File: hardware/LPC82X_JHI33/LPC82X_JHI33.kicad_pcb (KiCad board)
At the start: 2 copper layers, 23.6 x 23.5 mm, 24 parts, among them J1 LPC82XJHI33_LEFT, J2 LPC82XJHI33_RIGHT, J3 JTAG_2X05, U1 LPC824M201JHI33, Y1 12MHz

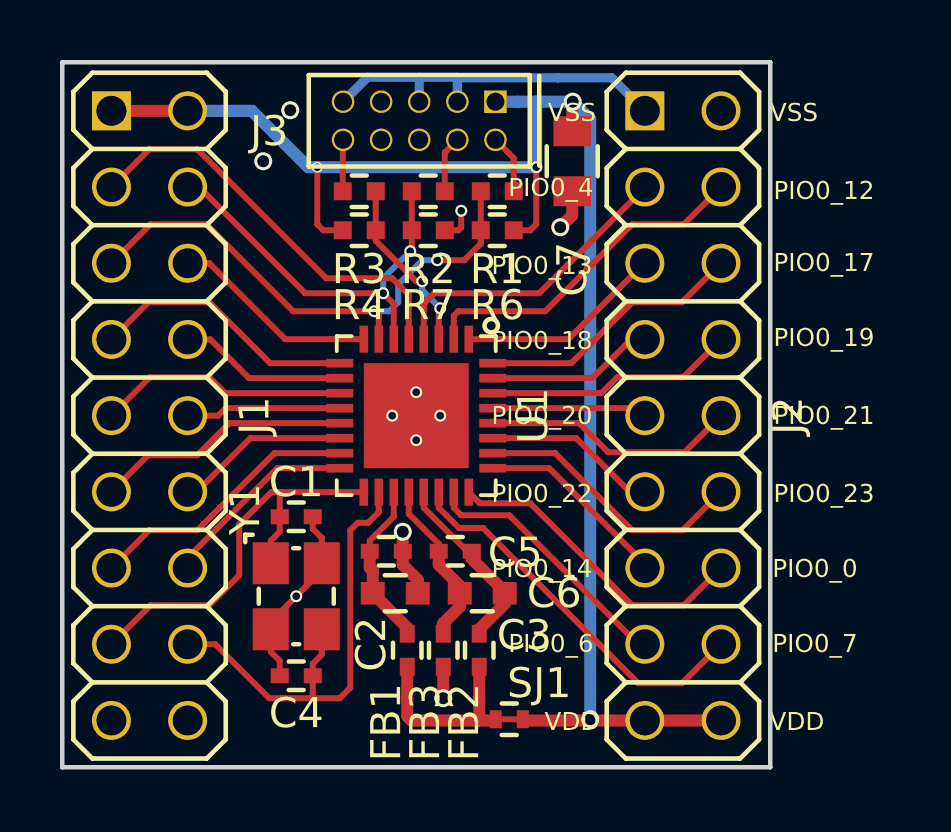
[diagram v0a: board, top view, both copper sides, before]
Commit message: silk placement completed
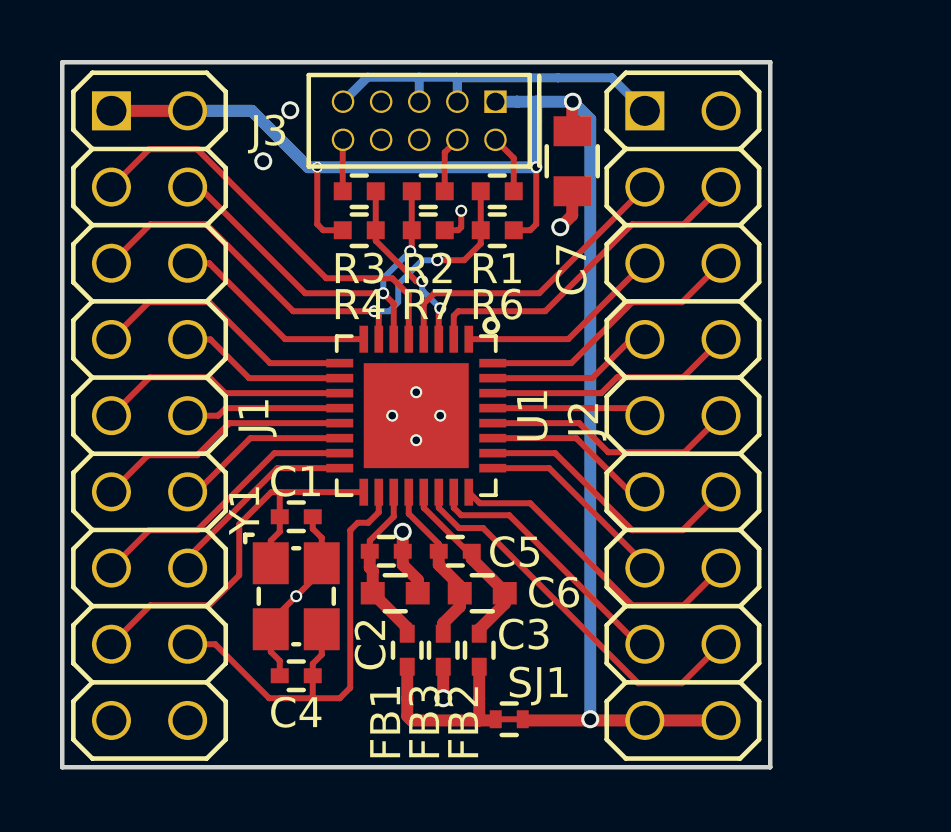
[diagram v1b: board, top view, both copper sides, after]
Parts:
- moved N2 6.30 mm to (87.7, 117.0)
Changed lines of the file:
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@@
     (tags "LPC82XJHI33 breakout right")
     (attr virtual)
-    (fp_text reference J2 (at 0 -3.5 270) (layer F.SilkS)
+    (fp_text reference J2 (at 0.12 3.29 270) (layer F.SilkS)
       (effects (font (size 1 1) (thickness 0.15)))
     )
@@
       (effects (font (size 1 1) (thickness 0.15)))
     )
-    (fp_text user VSS (at -10.1 -3.7) (layer F.SilkS)
-      (effects (font (size 0.6 0.6) (thickness 0.12)))
-    )
-    (fp_text user PIO0_12 (at -7.5 -4.7) (layer F.SilkS)
-      (effects (font (size 0.6 0.6) (thickness 0.12)))
-    )
-    (fp_text user PIO0_17 (at -5.1 -4.7) (layer F.SilkS)
-      (effects (font (size 0.6 0.6) (thickness 0.12)))
-    )
-    (fp_text user PIO0_19 (at -2.6 -4.7) (layer F.SilkS)
-      (effects (font (size 0.6 0.6) (thickness 0.12)))
-    )
-    (fp_text user PIO0_21 (at 0 -4.7) (layer F.SilkS)
-      (effects (font (size 0.6 0.6) (thickness 0.12)))
-    )
-    (fp_text user PIO0_23 (at 2.6 -4.7) (layer F.SilkS)
-      (effects (font (size 0.6 0.6) (thickness 0.12)))
-    )
-    (fp_text user PIO0_0 (at 5.1 -4.4) (layer F.SilkS)
-      (effects (font (size 0.6 0.6) (thickness 0.12)))
-    )
-    (fp_text user PIO0_7 (at 7.6 -4.4) (layer F.SilkS)
-      (effects (font (size 0.6 0.6) (thickness 0.12)))
-    )
-    (fp_text user VDD (at 10.2 -3.8) (layer F.SilkS)
-      (effects (font (size 0.6 0.6) (thickness 0.12)))
-    )
-    (fp_text user VDD (at 10.2 3.7) (layer F.SilkS)
-      (effects (font (size 0.6 0.6) (thickness 0.12)))
-    )
-    (fp_text user PIO0_6 (at 7.6 4.4) (layer F.SilkS)
-      (effects (font (size 0.6 0.6) (thickness 0.12)))
-    )
-    (fp_text user PIO0_14 (at 5.1 4.7) (layer F.SilkS)
-      (effects (font (size 0.6 0.6) (thickness 0.12)))
-    )
-    (fp_text user PIO0_22 (at 2.6 4.7) (layer F.SilkS)
-      (effects (font (size 0.6 0.6) (thickness 0.12)))
-    )
-    (fp_text user PIO0_20 (at 0 4.7) (layer F.SilkS)
-      (effects (font (size 0.6 0.6) (thickness 0.12)))
-    )
-    (fp_text user PIO0_18 (at -2.5 4.7) (layer F.SilkS)
-      (effects (font (size 0.6 0.6) (thickness 0.12)))
-    )
-    (fp_text user PIO0_13 (at -5 4.7) (layer F.SilkS)
-      (effects (font (size 0.6 0.6) (thickness 0.12)))
-    )
-    (fp_text user PIO0_4 (at -7.6 4.4) (layer F.SilkS)
-      (effects (font (size 0.6 0.6) (thickness 0.12)))
-    )
-    (fp_text user VSS (at -10.1 3.7) (layer F.SilkS)
-      (effects (font (size 0.6 0.6) (thickness 0.12)))
+    (fp_text user PIO0_12 (at -6.28 4.19 180) (layer B.SilkS)
+      (effects (font (size 0.6 0.6) (thickness 0.12)) (justify mirror))
+    )
+    (fp_text user PIO0_17 (at -3.78 4.19 180) (layer B.SilkS)
+      (effects (font (size 0.6 0.6) (thickness 0.12)) (justify mirror))
+    )
+    (fp_text user PIO0_19 (at -1.28 4.19 180) (layer B.SilkS)
+      (effects (font (size 0.6 0.6) (thickness 0.12)) (justify mirror))
+    )
+    (fp_text user PIO0_21 (at 1.32 4.19 180) (layer B.SilkS)
+      (effects (font (size 0.6 0.6) (thickness 0.12)) (justify mirror))
+    )
+    (fp_text user PIO0_23 (at 3.82 4.19 180) (layer B.SilkS)
+      (effects (font (size 0.6 0.6) (thickness 0.12)) (justify mirror))
+    )
+    (fp_text user PIO0_0 (at 6.42 3.89 180) (layer B.SilkS)
+      (effects (font (size 0.6 0.6) (thickness 0.12)) (justify mirror))
+    )
+    (fp_text user PIO0_7 (at 8.92 3.89 180) (layer B.SilkS)
+      (effects (font (size 0.6 0.6) (thickness 0.12)) (justify mirror))
+    )
+    (fp_text user VDD (at 10.2 3.69 180) (layer B.SilkS)
+      (effects (font (size 0.6 0.6) (thickness 0.12)) (justify mirror))
+    )
+    (fp_text user PIO0_6 (at 7.6 4.4 180) (layer B.SilkS)
+      (effects (font (size 0.6 0.6) (thickness 0.12)) (justify mirror))
+    )
+    (fp_text user PIO0_14 (at 5.1 4.7 180) (layer B.SilkS)
+      (effects (font (size 0.6 0.6) (thickness 0.12)) (justify mirror))
+    )
+    (fp_text user PIO0_22 (at 2.6 4.7 180) (layer B.SilkS)
+      (effects (font (size 0.6 0.6) (thickness 0.12)) (justify mirror))
+    )
+    (fp_text user PIO0_20 (at -0.38 4.49 180) (layer B.SilkS)
+      (effects (font (size 0.6 0.6) (thickness 0.12)) (justify mirror))
+    )
+    (fp_text user PIO0_18 (at -2.5 4.7 180) (layer B.SilkS)
+      (effects (font (size 0.6 0.6) (thickness 0.12)) (justify mirror))
+    )
+    (fp_text user PIO0_13 (at -5 4.7 180) (layer B.SilkS)
+      (effects (font (size 0.6 0.6) (thickness 0.12)) (justify mirror))
+    )
+    (fp_text user PIO0_4 (at -7.6 4.4 180) (layer B.SilkS)
+      (effects (font (size 0.6 0.6) (thickness 0.12)) (justify mirror))
+    )
+    (fp_text user VSS (at -10.1 3.7 180) (layer B.SilkS)
+      (effects (font (size 0.6 0.6) (thickness 0.12)) (justify mirror))
     )
     (fp_line (start 9.525 2.54) (end 10.795 2.54) (layer F.SilkS) (width 0.1524))
@@
       (effects (font (size 0.6 0.6) (thickness 0.12)) (justify mirror))
     )
-    (fp_text user PIO0_26 (at 0 -4.7 180) (layer B.SilkS)
+    (fp_text user PIO0_26 (at -0.28 -4.49 180) (layer B.SilkS)
       (effects (font (size 0.6 0.6) (thickness 0.12)) (justify mirror))
     )
@@
       (effects (font (size 0.6 0.6) (thickness 0.12)) (justify mirror))
     )
-    (fp_text user VSS (at 10.2 -3.7 180) (layer B.SilkS)
+    (fp_text user VSS (at 10.22 -3.49 180) (layer B.SilkS)
       (effects (font (size 0.6 0.6) (thickness 0.12)) (justify mirror))
     )
@@
   )
   (module SquantorLabels:Label_version (layer B.Cu)
-    (at 87.7 110.7 180)
+    (at 87.7 117 180)
     (fp_text reference N2 (at 0 -1.4 180) (layer B.Fab) hide
       (effects (font (size 1 1) (thickness 0.15)) (justify mirror))
